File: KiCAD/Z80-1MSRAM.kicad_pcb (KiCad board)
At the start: 2 copper layers, 99.1 x 74.9 mm, 27 parts, among them J1 SBC8080 BUS, J2 I/O ADDR SEL, U1 74HC02, U2 74HC74, U3 74HC139, U4 74HC04, U5 74HC00, U6 628128, U7 28C256

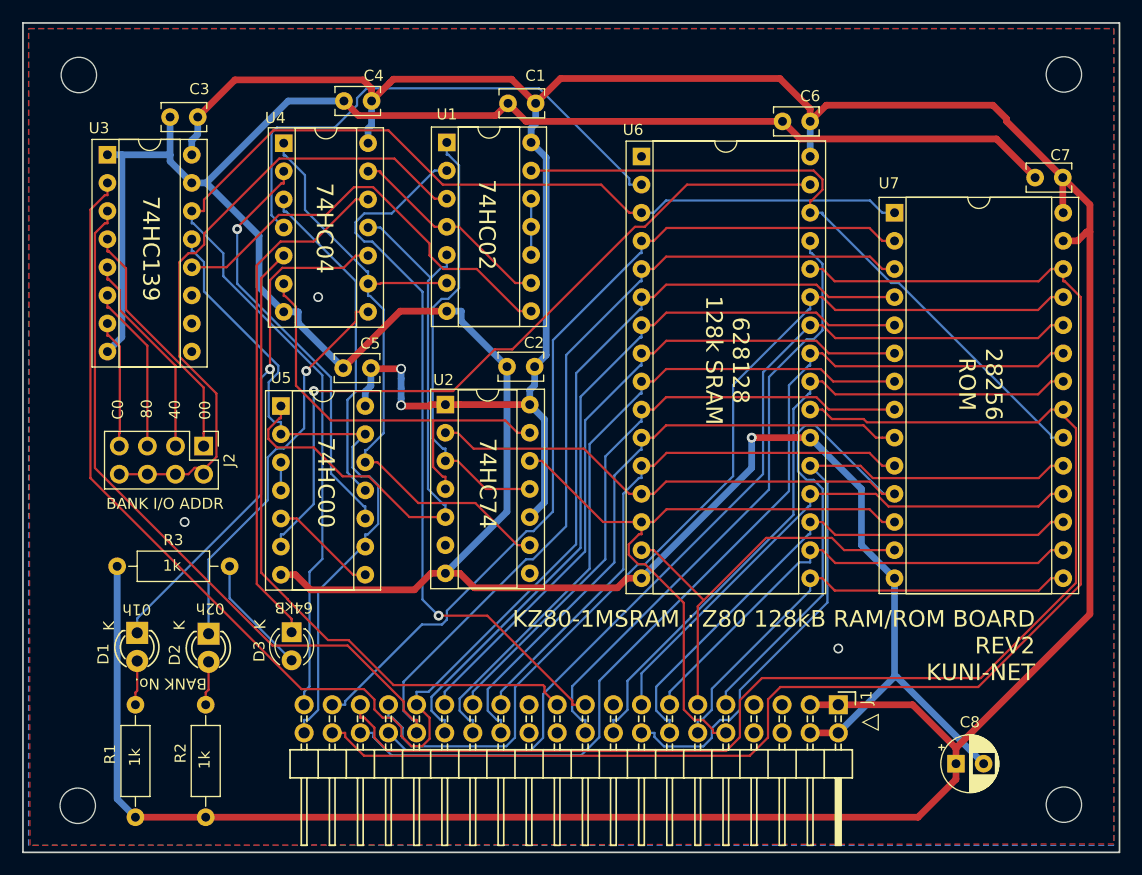
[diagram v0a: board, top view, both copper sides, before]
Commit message: REV3 基板関係 試作バージョン
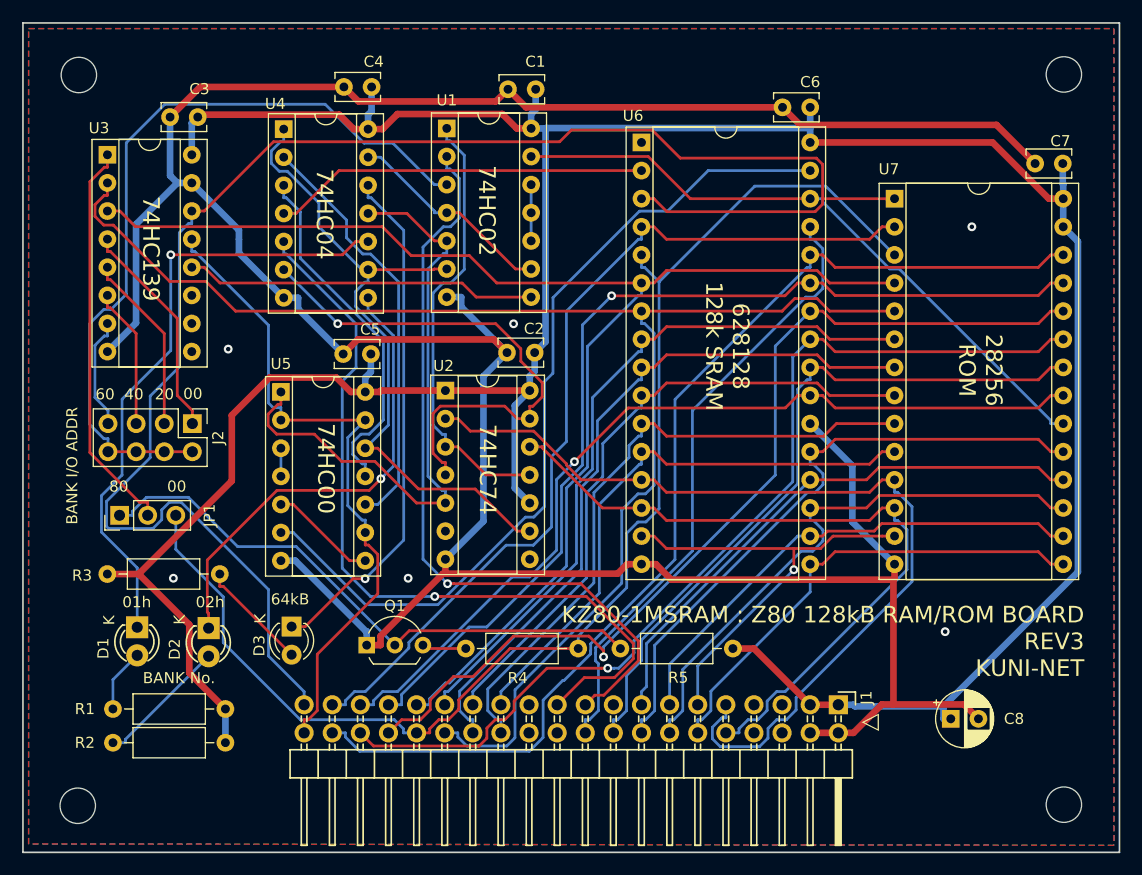
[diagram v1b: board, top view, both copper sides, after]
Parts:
- added JP1: A7_Jumper, Connector_PinHeader_2.54mm:PinHeader_1x03_P2.54mm_Vertical, F.Cu at (110.3, 108.0)
- added Q1: 2SC1815, Package_TO_SOT_THT:TO-92L_Inline_Wide, F.Cu at (132.7, 119.7)
- added R4: 100k, Resistor_THT:R_Axial_DIN0207_L6.3mm_D2.5mm_P10.16mm_Horizontal, F.Cu at (141.6, 120.0)
- added R5: 1k, Resistor_THT:R_Axial_DIN0207_L6.3mm_D2.5mm_P10.16mm_Horizontal, F.Cu at (155.6, 120.0)
- R1, R2: footprint Resistors_THT:R_Axial_DIN0207_L6.3mm_D2.5mm_P10.16mm_Horizontal -> Resistor_THT:R_Axial_DIN0207_L6.3mm_D2.5mm_P10.16mm_Horizontal
- moved R1 12.7 mm to (119.9, 125.5), turned to 180 degrees
- moved R2 6.96 mm to (119.9, 128.5), turned to 180 degrees
- moved C8 4.08 mm to (185.4, 126.4)
- moved J2 2.27 mm to (116.9, 99.7)
- moved C1 1.27 mm to (147.9, 69.5)
- moved C2 1.27 mm to (147.8, 93.3)
- moved C4 1.27 mm to (133.1, 69.3)
- moved U2 1.27 mm to (139.8, 96.7)
- moved U4 1.27 mm to (125.2, 73.1)
- moved C5 1.27 mm to (133.0, 93.4)
- moved C6 1.27 mm to (172.7, 71.1)
- moved C7 1.27 mm to (195.5, 76.2)
- moved U1 1.27 mm to (139.9, 73.0)
- moved U5 1.27 mm to (124.9, 96.8)
- moved U6 1.27 mm to (157.5, 74.3)
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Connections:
- J1 pad 32: /A7 -> A7
- U3 pad 1: GND -> ADDR_SEL
- U3 pad 2: /A6 -> /A5
- U3 pad 3: /A7 -> /A6
- U6 pad 5: /A7 -> A7
- U7 pad 3: /A7 -> A7
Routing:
- net /A7: track 139.7 -> 0.00 mm
- net A7: track 0.00 -> 120.1 mm
- net /A5: track 69.3 -> 132.5 mm
- net VCC: track 341.4 -> 281.4 mm, vias 2 -> 0
- net Net-(JP1-Pad1): track 0.00 -> 52.9 mm
- net /A10: track 116.0 -> 80.0 mm, vias 0 -> 1
- net ADDR_SEL: track 0.00 -> 36.0 mm
- net /A13: track 130.1 -> 98.1 mm
- net /A14: track 121.4 -> 151.6 mm
- net /A6: track 142.7 -> 122.3 mm
- net /MEMA16: track 48.4 -> 33.9 mm
- net Net-(J2-Pad2): track 59.1 -> 71.6 mm
- net RES: track 61.5 -> 72.0 mm, vias 0 -> 1
- net /MEMA15: track 68.0 -> 77.4 mm, vias 1 -> 0
- net Net-(D1-Pad1): track 46.6 -> 55.9 mm
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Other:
- net class BOLD: clearance 0.2032 -> 0.2; trace_width 0.6096 -> 0.6; via_dia 0.889 -> 0.8; via_drill 0.6096 -> 0.4
- net class Default: clearance 0.2032 -> 0.2; trace_width 0.2032 -> 0.25; via_dia 0.889 -> 0.8; via_drill 0.6096 -> 0.4
- rule trace_clearance: 0.2032 -> 0.2
- rule trace_min: 0.2032 -> 0.2
- rule via_min_drill: 0.6096 -> 0.4
- rule via_min_size: 0.889 -> 0.8
- board text added: "20"
- board text added: "60"
- board text added: "KZ80-1MSRAM : Z80 128kB RAM/ROM BOARD REV3 KUNI-NET"
- board text removed: "1k"
- board text removed: "C0"
- board text removed: "KZ80-1MSRAM : Z80 128kB RAM/ROM BOARD REV2 KUNI-NET"
